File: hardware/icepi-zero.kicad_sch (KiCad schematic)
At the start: 25 parts, among them J1 Conn_02x20_Counter_Clockwise, SW1 SW_Push, U3 ECP5U_12_CABGA256

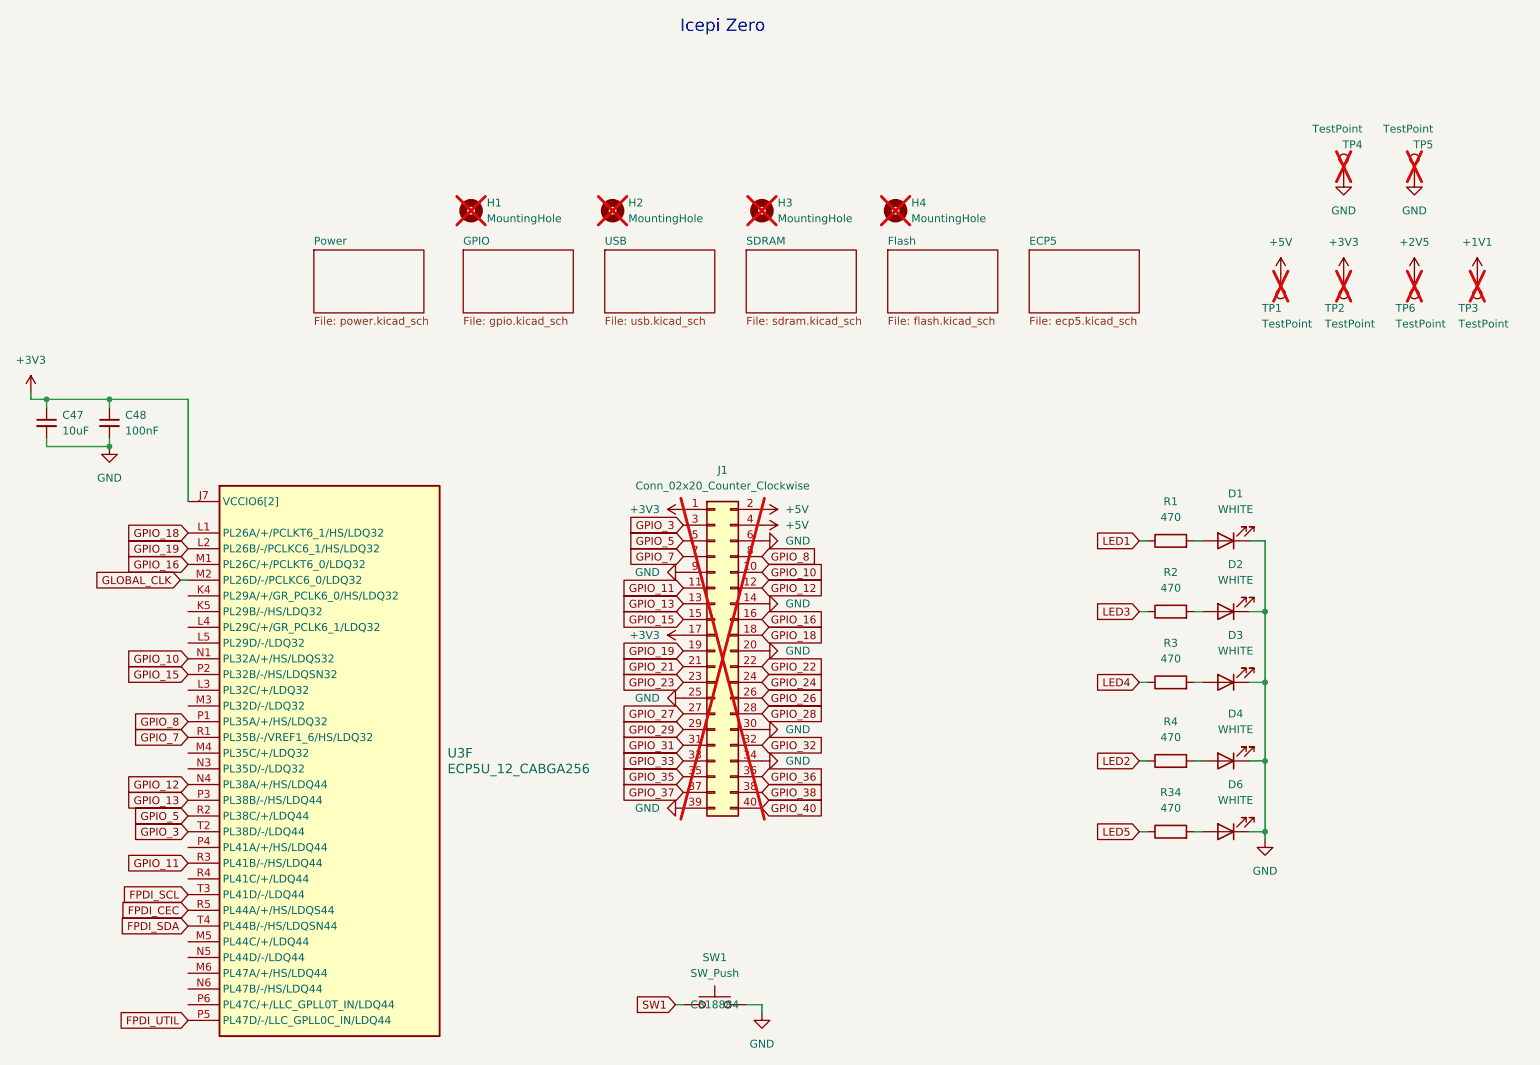
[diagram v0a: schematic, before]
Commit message: Final revision
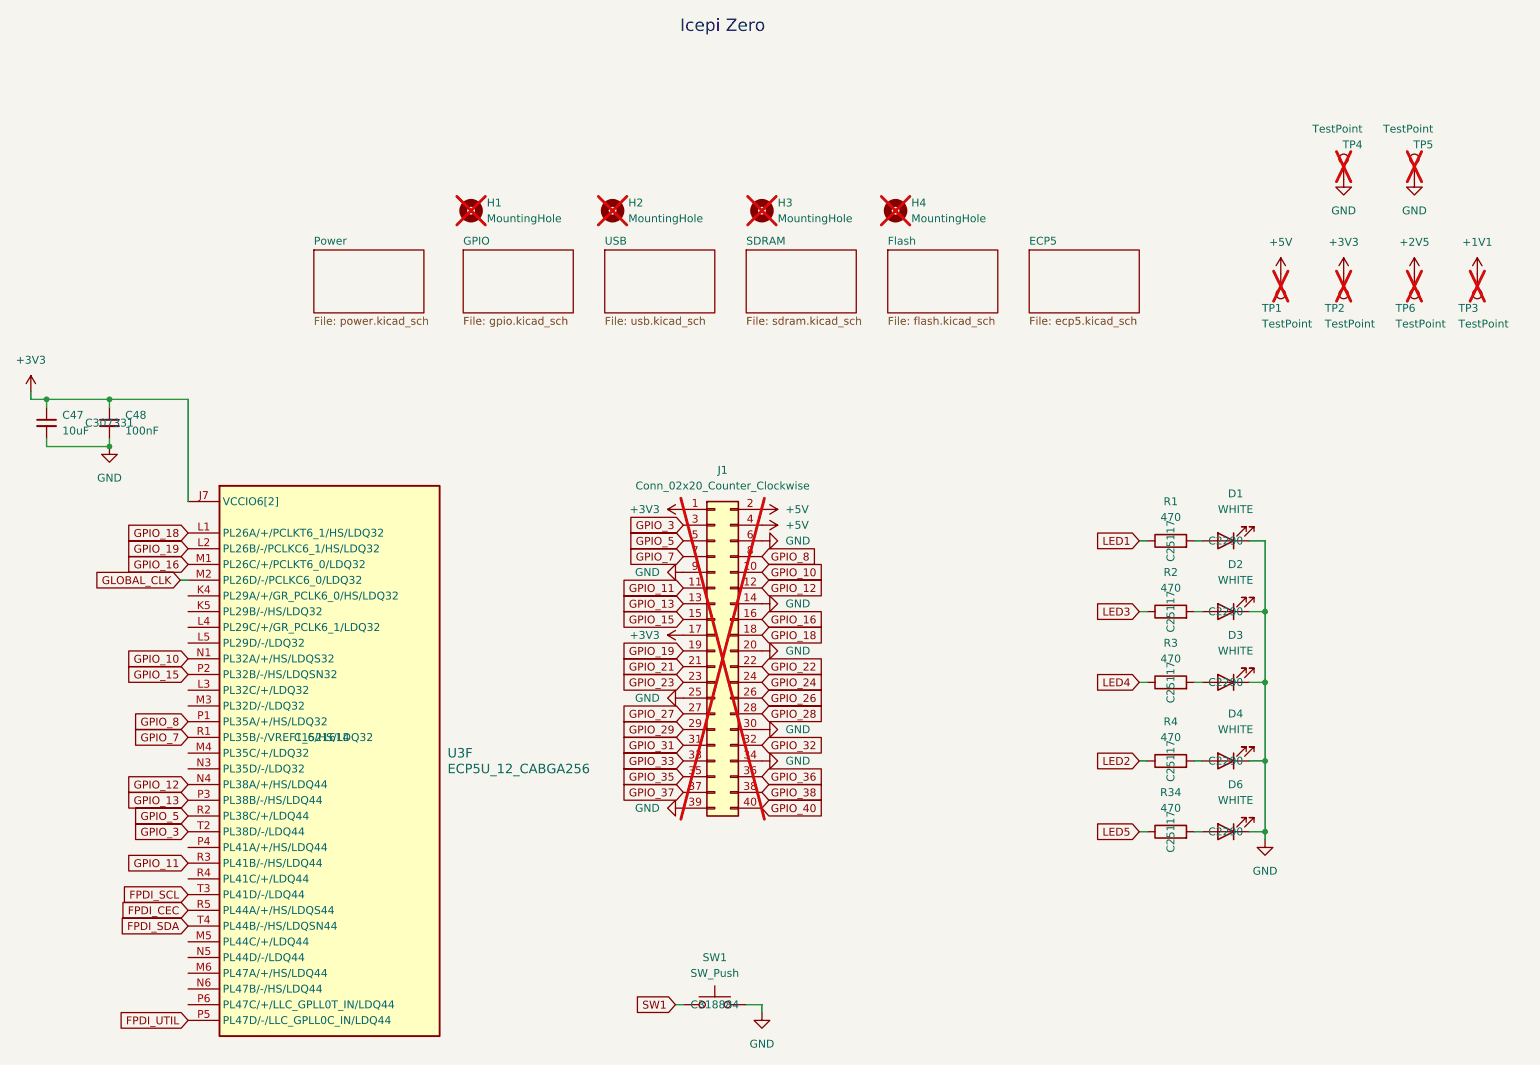
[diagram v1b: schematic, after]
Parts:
- C48: JLCPCB Part # C307331 -> (none); LCSC Part # (none) -> C307331
- D1, D2, D3, D4, D6: JLCPCB Part # C2290 -> (none); LCSC Part # (none) -> C2290
- R1, R2, R3, R34, R4: JLCPCB Part # C25117 -> (none); LCSC Part # (none) -> C25117
- SW1: JLCPCB Part # C318884 -> (none); LCSC Part # (none) -> C318884
- U3: JLCPCB Part # C1521614 -> (none); LCSC Part # (none) -> C1521614
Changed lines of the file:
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@@
 			)
 		)
-		(property "JLCPCB Part #" "C2290"
+		(property "LCSC Part #" "C2290"
 			(at 217.17 101.6 0)
 			(effects
@@
 					(size 1.27 1.27)
 				)
-				(hide yes)
 			)
 		)
@@
 			)
 		)
-		(property "JLCPCB Part #" "C25117"
+		(property "LCSC Part #" "C25117"
 			(at 208.28 113.03 0)
 			(effects
@@
 					(size 1.27 1.27)
 				)
-				(hide yes)
 			)
 		)
@@
 			)
 		)
-		(property "JLCPCB Part #" "C25117"
+		(property "LCSC Part #" "C25117"
 			(at 208.28 148.59 0)
 			(effects
@@
 					(size 1.27 1.27)
 				)
-				(hide yes)
 			)
 		)
@@
 			)
 		)
-		(property "JLCPCB Part #" "C25117"
+		(property "LCSC Part #" "C25117"
 			(at 208.28 101.6 0)
 			(effects
@@
 					(size 1.27 1.27)
 				)
-				(hide yes)
 			)
 		)
@@
 			)
 		)
-		(property "JLCPCB Part #" "C2290"
+		(property "LCSC Part #" "C2290"
 			(at 217.17 113.03 0)
 			(effects
@@
 					(size 1.27 1.27)
 				)
-				(hide yes)
 			)
 		)
@@
 			)
 		)
-		(property "JLCPCB Part #" ""
-			(at 118.11 48.26 0)
-			(effects
-				(font
-					(size 1.27 1.27)
-				)
-				(hide yes)
-			)
-		)
 		(instances
 			(project "icepi-zero"
@@
 			)
 		)
-		(property "JLCPCB Part #" ""
-			(at 134.62 119.38 0)
-			(effects
-				(font
-					(size 1.27 1.27)
-				)
-				(hide yes)
-			)
-		)
 		(pin "23"
 		)
@@
 			)
 		)
-		(property "JLCPCB Part #" ""
-			(at 163.83 48.26 0)
-			(effects
-				(font
-					(size 1.27 1.27)
-				)
-				(hide yes)
-			)
-		)
 		(instances
 			(project "icepi-zero"
@@
 			)
 		)
-		(property "JLCPCB Part #" "C25117"
+		(property "LCSC Part #" "C25117"
 			(at 208.28 137.16 0)
 			(effects
@@
 					(size 1.27 1.27)
 				)
-				(hide yes)
 			)
 		)
@@
 			)
 		)
-		(property "JLCPCB Part #" "C25117"
+		(property "LCSC Part #" "C25117"
 			(at 208.28 124.46 0)
 			(effects
@@
 					(size 1.27 1.27)
 				)
-				(hide yes)
 			)
 		)
@@
 			)
 		)
-		(property "JLCPCB Part #" ""
-			(at 142.24 48.26 0)
-			(effects
-				(font
-					(size 1.27 1.27)
-				)
-				(hide yes)
-			)
-		)
 		(instances
 			(project "icepi-zero"
@@
 			)
 		)
-		(property "JLCPCB Part #" ""
-			(at 95.25 48.26 0)
-			(effects
-				(font
-					(size 1.27 1.27)
-				)
-				(hide yes)
-			)
-		)
 		(instances
 			(project ""
@@
 			)
 		)
-		(property "JLCPCB Part #" "C2290"
+		(property "LCSC Part #" "C2290"
 			(at 217.17 124.46 0)
 			(effects
@@
 					(size 1.27 1.27)
 				)
-				(hide yes)
 			)
 		)
@@
 			)
 		)
-		(property "JLCPCB Part #" "C1521614"
+		(property "LCSC Part #" "C1521614"
 			(at 71.12 133.35 0)
 			(effects
@@
 					(size 1.27 1.27)
 				)
-				(hide yes)
 			)
 		)
@@
 			)
 		)
-		(property "JLCPCB Part #" "C307331 "
+		(property "LCSC Part #" "C307331 "
 			(at 36.83 82.55 0)
 			(effects
@@
 					(size 1.27 1.27)
 				)
-				(hide yes)
 			)
 		)
@@
 			)
 		)
-		(property "JLCPCB Part #" "C2290"
+		(property "LCSC Part #" "C2290"
 			(at 217.17 137.16 0)
 			(effects
@@
 					(size 1.27 1.27)
 				)
-				(hide yes)
 			)
 		)
@@
 			)
 		)
-		(property "JLCPCB Part #" "C2290"
+		(property "LCSC Part #" "C2290"
 			(at 217.17 148.59 0)
 			(effects
@@
 					(size 1.27 1.27)
 				)
-				(hide yes)
 			)
 		)
@@
 			)
 		)
-		(property "JLCPCB Part #" "C318884"
+		(property "LCSC Part #" "C318884"
 			(at 134.62 176.53 0)
 			(effects

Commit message: Last checks
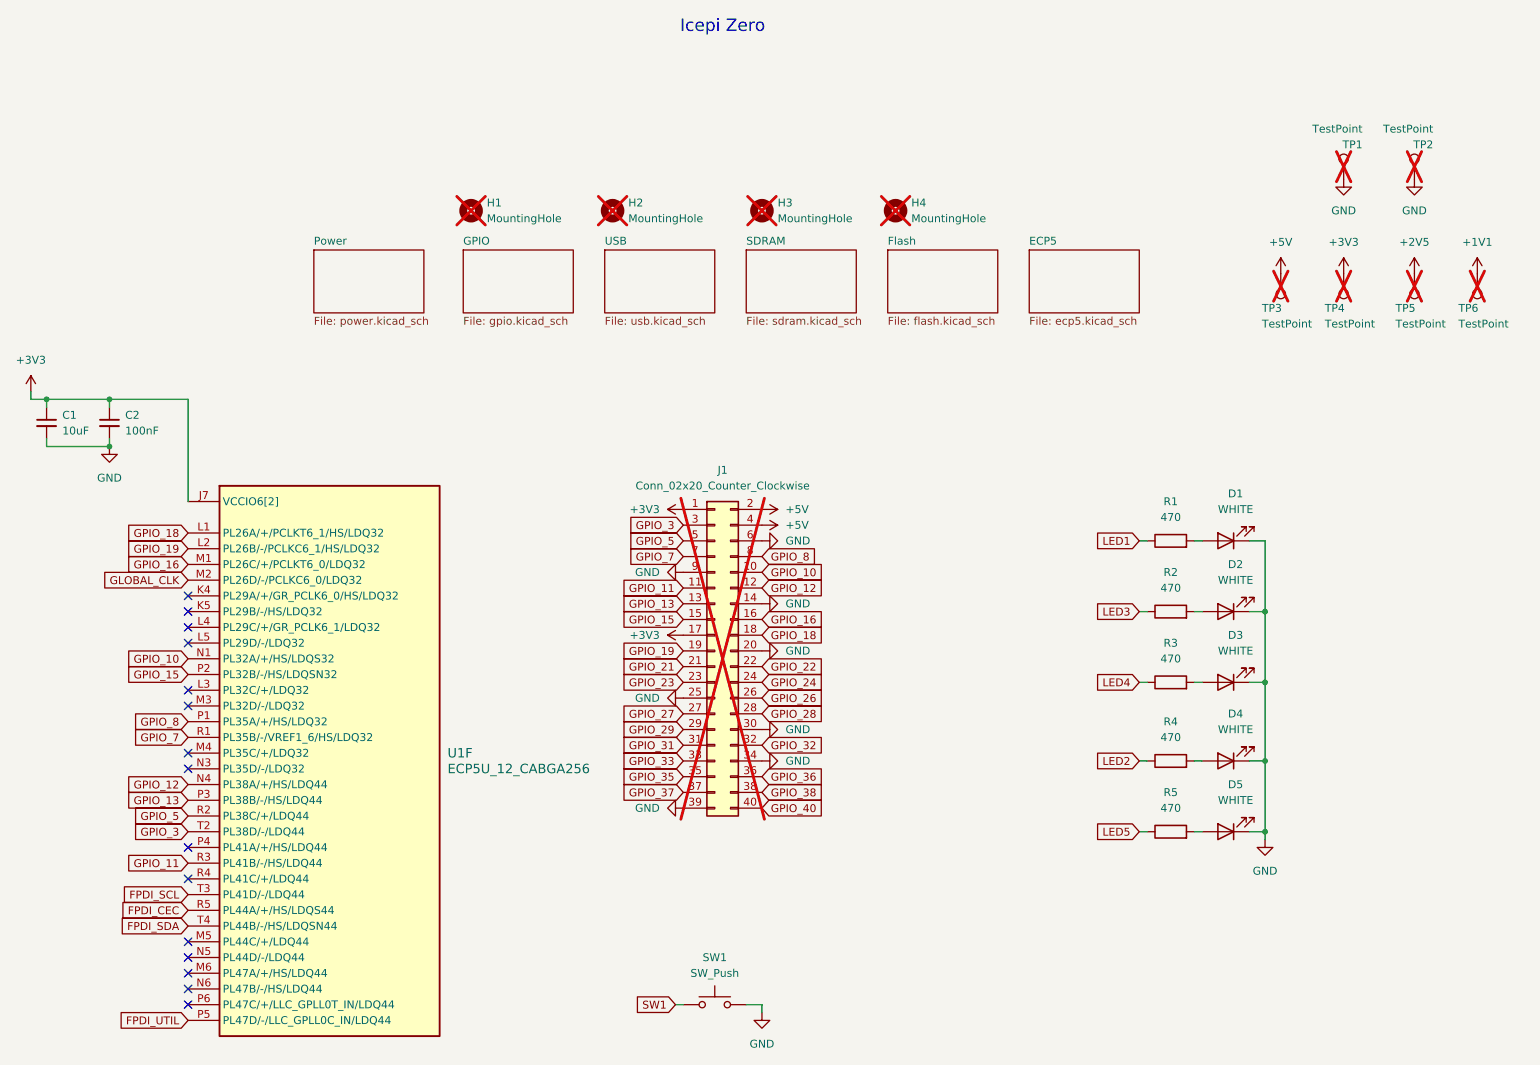
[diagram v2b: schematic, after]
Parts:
- C1: renamed from C47; LCSC Part # (none) -> C19702
- renumbered C48 to C2, D6 to D5, R34 to R5, TP4 to TP1, TP5 to TP2, TP1 to TP3, TP2 to TP4, TP6 to TP5, TP3 to TP6, U3 to U1
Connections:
- no-connect marks 0 -> 15

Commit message: Final production files
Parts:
- H1, H2, H3, H4: footprint MountingHole:MountingHole_2.5mm -> MountingHole:MountingHole_2.7mm_M2.5
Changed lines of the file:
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@@
 			)
 		)
-		(property "Footprint" "MountingHole:MountingHole_2.5mm"
+		(property "Footprint" "MountingHole:MountingHole_2.7mm_M2.5"
 			(at 118.11 48.26 0)
 			(effects
@@
 			)
 		)
-		(property "Footprint" "MountingHole:MountingHole_2.5mm"
+		(property "Footprint" "MountingHole:MountingHole_2.7mm_M2.5"
 			(at 163.83 48.26 0)
 			(effects
@@
 			)
 		)
-		(property "Footprint" "MountingHole:MountingHole_2.5mm"
+		(property "Footprint" "MountingHole:MountingHole_2.7mm_M2.5"
 			(at 142.24 48.26 0)
 			(effects
@@
 			)
 		)
-		(property "Footprint" "MountingHole:MountingHole_2.5mm"
+		(property "Footprint" "MountingHole:MountingHole_2.7mm_M2.5"
 			(at 95.25 48.26 0)
 			(effects
